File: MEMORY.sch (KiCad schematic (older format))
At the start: 77 parts, among them U2 MCIMX7D7DVM10SC

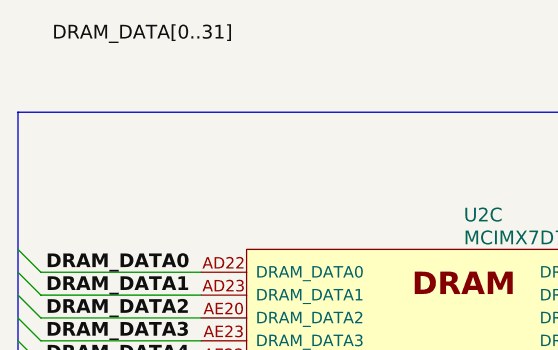
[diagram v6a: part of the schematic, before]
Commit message: modified adui circuit
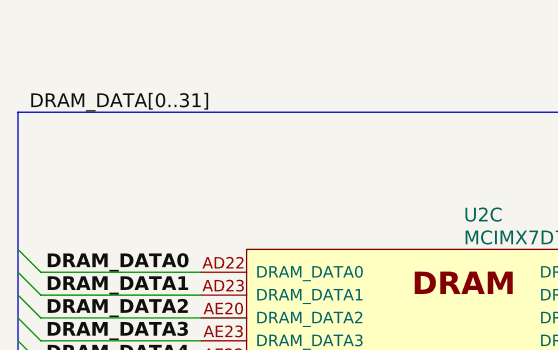
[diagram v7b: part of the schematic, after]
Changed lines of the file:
@@
 LIBS:mtfc8gacaeam-1m_wt
 LIBS:sn74avc2t244
-LIBS:lsm9ds1
+LIBS:WM8960CGEFL
 LIBS:3210retro-cache
 EELAYER 25 0
@@
 Wire Bus Line
 	6600 1350 6600 4000
-Text Label 1800 800  0    60   ~ 0
+Text Label 1700 1100 0    60   ~ 0
 DRAM_DATA[0..31]
 Text Label 5600 1350 0    60   ~ 0
